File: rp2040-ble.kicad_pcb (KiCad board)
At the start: 2 copper layers, 41 parts, among them J1 Conn_01x15, J2 Conn_01x15, J3 USB_B_Micro, J4 Conn_01x03, SW1 SW_Push, SW2 SW_Push, U1 RP2040, U2 W25Q128JVS, U3 HM-BT4502, U4 NCP1117DT33G, Y1 ABLS-12.000MHZ-B4-T

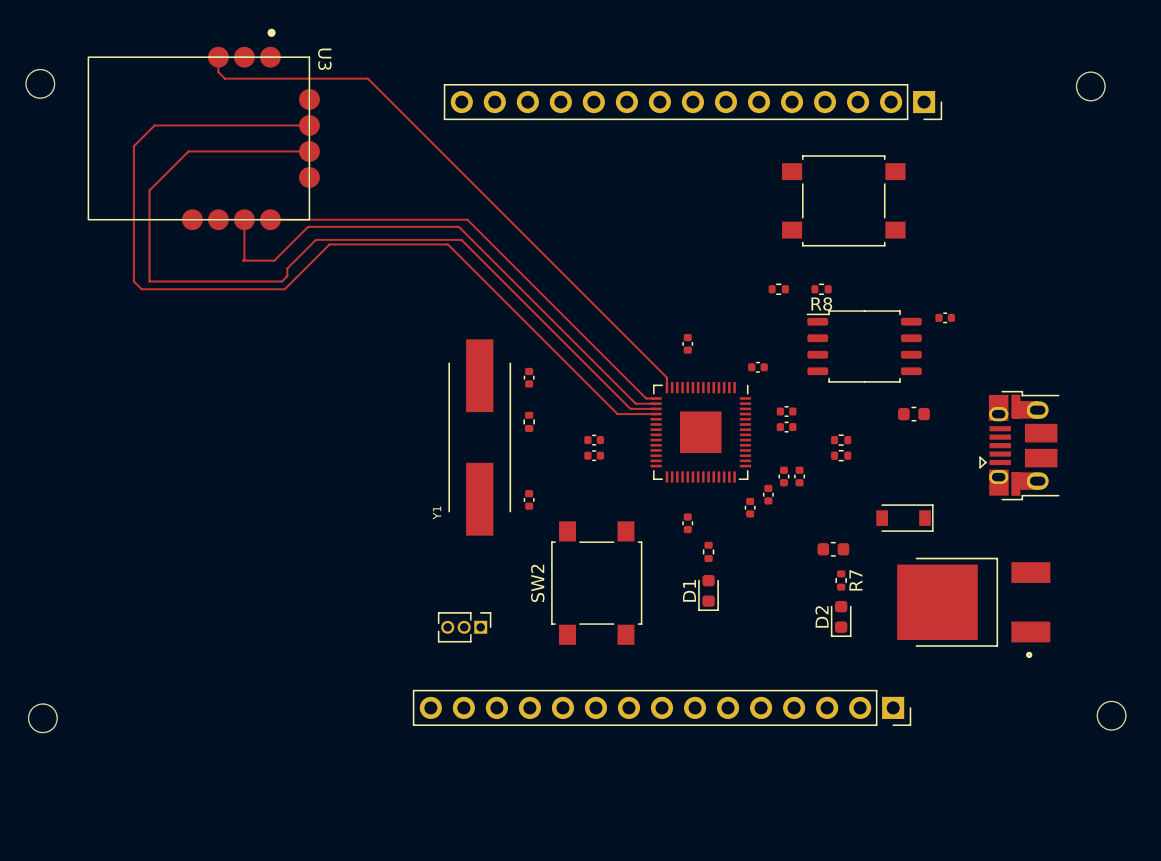
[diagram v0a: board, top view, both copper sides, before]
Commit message: PCB roouting
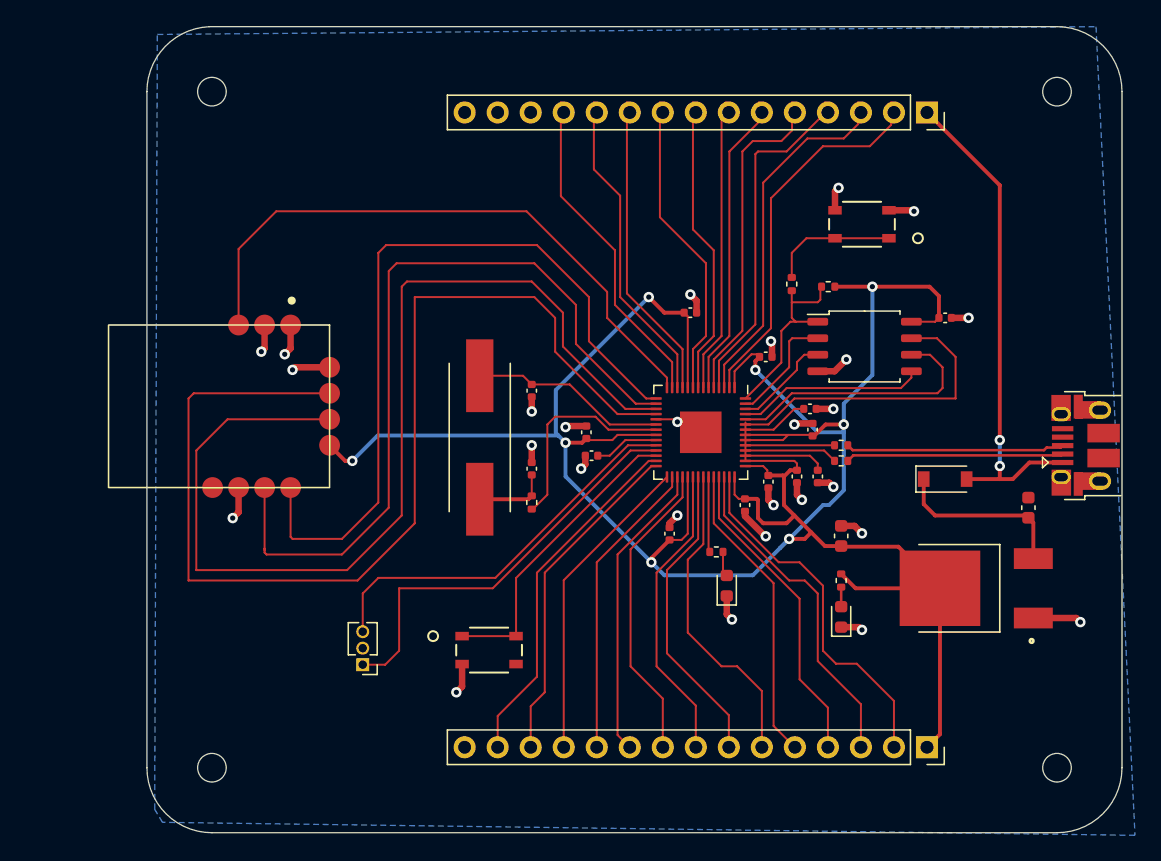
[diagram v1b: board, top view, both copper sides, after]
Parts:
- SW1, SW2: value SW_Push -> PTS810_SJK_250_SMTR_LFS; footprint Button_Switch_SMD:SW_SPST_B3S-1000 -> PTS810:PTS810 SJK 250 SMTR LFS
- moved U3 20.7 mm to (95.5, 96.2)
- moved H4 13.5 mm to (95.0, 124.0)
- moved H2 13.2 mm to (95.0, 72.0)
- moved C15 11.4 mm to (157.8, 104.0), turned to 90 degrees
- moved SW2 9.75 mm to (116.3, 115.0), turned to 0 degrees
- moved J4 9.52 mm to (106.6, 116.1), turned to 180 degrees
- moved C10 8.40 mm to (119.6, 95.0)
- moved C13 7.00 mm to (119.6, 101.0)
- moved R4 6.20 mm to (119.6, 103.6)
- moved H1 5.80 mm to (160.0, 124.0)
- moved J3 4.80 mm to (162.2, 99.2)
- moved D3 4.39 mm to (151.4, 101.8), turned to 0 degrees
- moved J2 3.99 mm to (150.0, 122.4)
- moved H3 2.63 mm to (160.0, 72.0)
- moved C3 2.41 mm to (131.8, 89.0), turned to 0 degrees
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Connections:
- J2 pad 1: /GPIO29 -> +3.3V
- J2 pad 2: +3.3V -> /GPIO29
- R6 pad 2: Net-(R6-Pad2) -> /USB_BOOT
- SW1 pad 1: GND -> /USB_BOOT
- SW1 pad 2: Net-(R6-Pad2) -> /USB_BOOT
- SW2 pad 1: GND -> /RUN
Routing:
- net +3.3V: track 0.00 -> 203.0 mm, vias 0 -> 8
- net GND: track 0.00 -> 49.9 mm, vias 0 -> 27
- net /VBUS: track 0.00 -> 38.4 mm, vias 0 -> 2
- net /SWD: track 0.00 -> 32.2 mm
- net /SWCLK: track 0.00 -> 30.2 mm
- net /GPIO0: track 0.00 -> 29.2 mm
- net /GPIO29: track 0.00 -> 27.9 mm
- net /GPIO1: track 0.00 -> 27.9 mm
- net /GPIO16: track 0.00 -> 27.4 mm
- net /GPIO2: track 0.00 -> 26.6 mm
- net /GPIO28: track 0.00 -> 25.8 mm
- net /GPIO17: track 0.00 -> 25.8 mm
- net /GPIO3: track 0.00 -> 25.7 mm
- net /GPIO10: track 0.00 -> 25.5 mm
- net /GPIO9: track 0.00 -> 24.6 mm
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- added copper zone on B.Cu, net GND
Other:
- board outline added: 75 x 62 mm
